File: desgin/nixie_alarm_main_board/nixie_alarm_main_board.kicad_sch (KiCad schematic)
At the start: 1 part, among them U1 ESP32-S3-WROOM-1

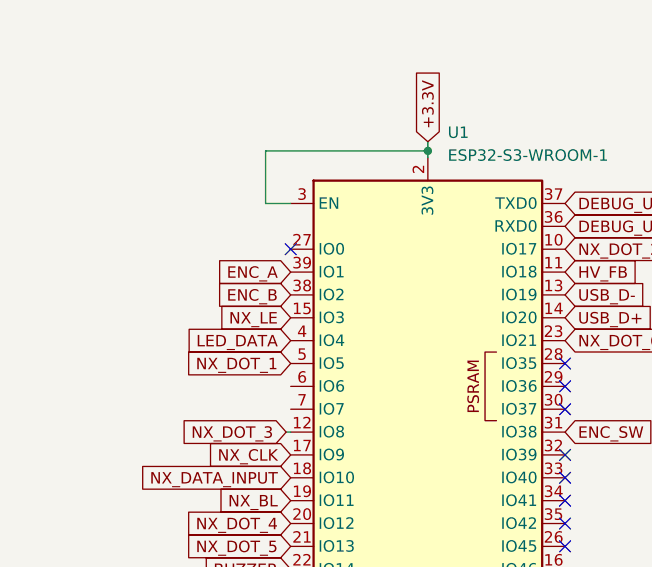
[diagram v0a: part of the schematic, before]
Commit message: copper border
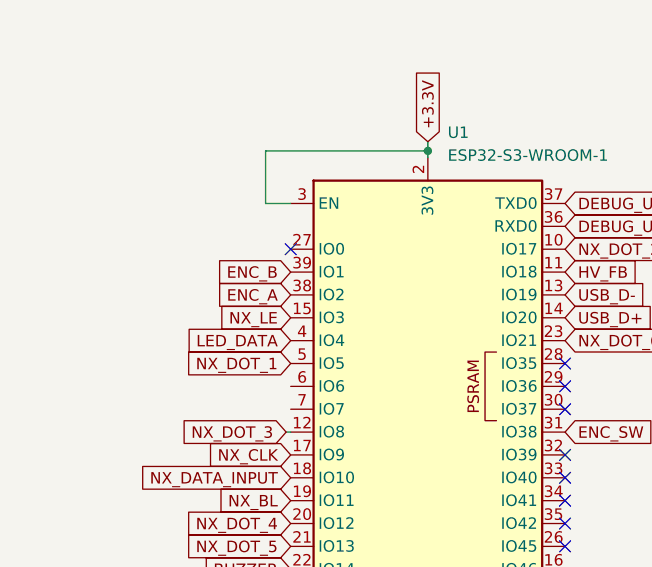
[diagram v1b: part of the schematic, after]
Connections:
- net ENC_A: now also U1.38 (IO2); no longer U1.39 (IO1)
- net ENC_B: now also U1.39 (IO1); no longer U1.38 (IO2)

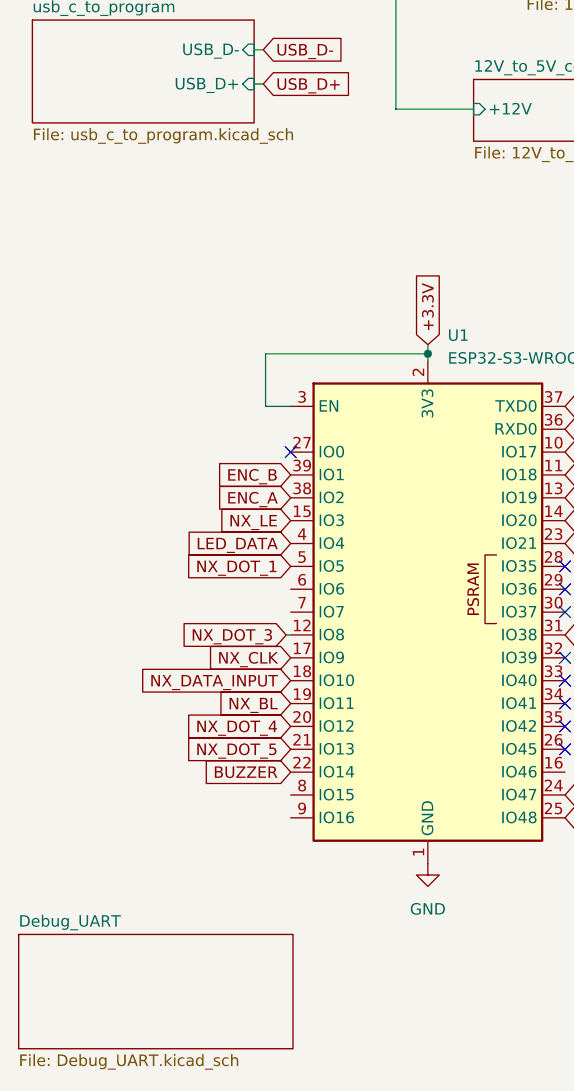
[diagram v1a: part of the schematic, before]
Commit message: little fixes
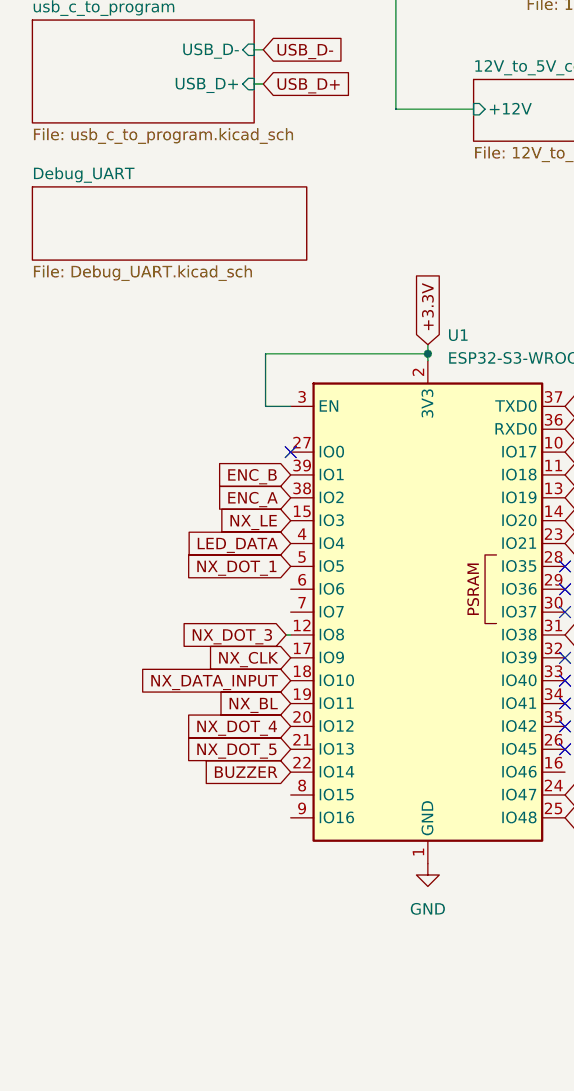
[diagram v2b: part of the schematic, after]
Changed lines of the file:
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@@
 	)
 	(sheet
-		(at 82.042 145.796)
-		(size 30.48 12.7)
+		(at 83.566 62.738)
+		(size 30.48 8.128)
 		(fields_autoplaced yes)
 		(stroke
@@
 		)
 		(property "Sheetname" "Debug_UART"
-			(at 82.042 145.0844 0)
+			(at 83.566 62.0264 0)
 			(effects
 				(font
@@
 		)
 		(property "Sheetfile" "Debug_UART.kicad_sch"
-			(at 82.042 159.0806 0)
+			(at 83.566 71.4506 0)
 			(effects
 				(font
